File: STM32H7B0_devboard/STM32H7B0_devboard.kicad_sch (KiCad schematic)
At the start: 20 parts, among them SW1 SW_SPDT, U1 STM32H7B0VBT6, Y1 25MHz, Y2 32.768KHz

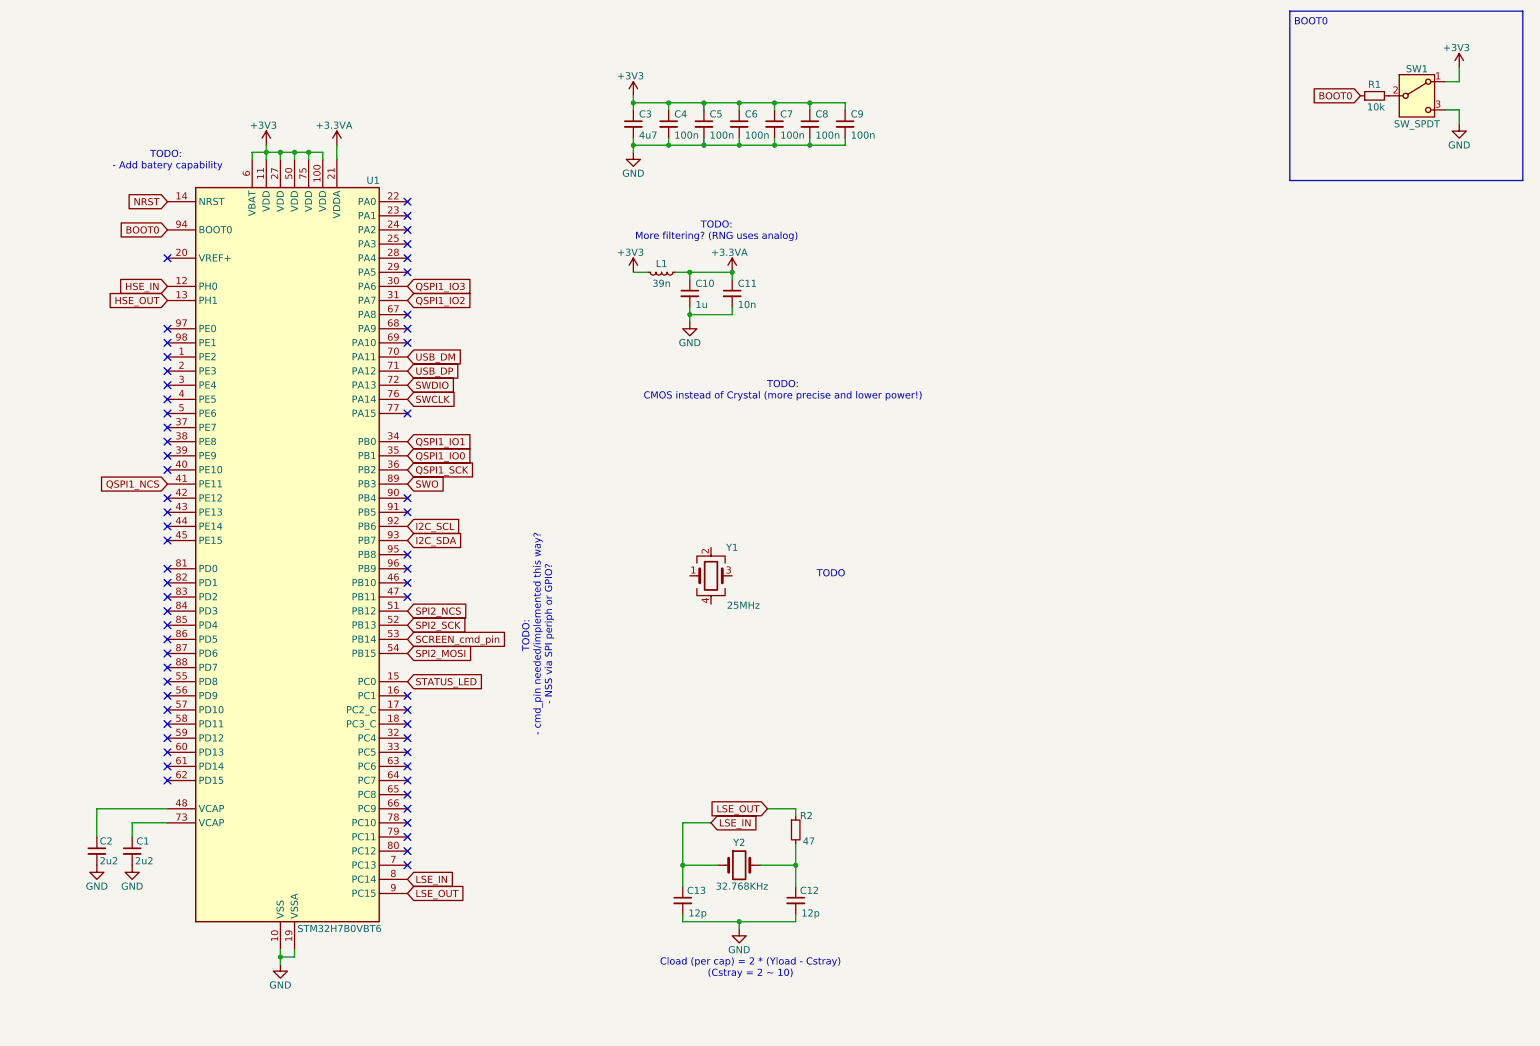
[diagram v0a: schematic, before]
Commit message: Schematic V0
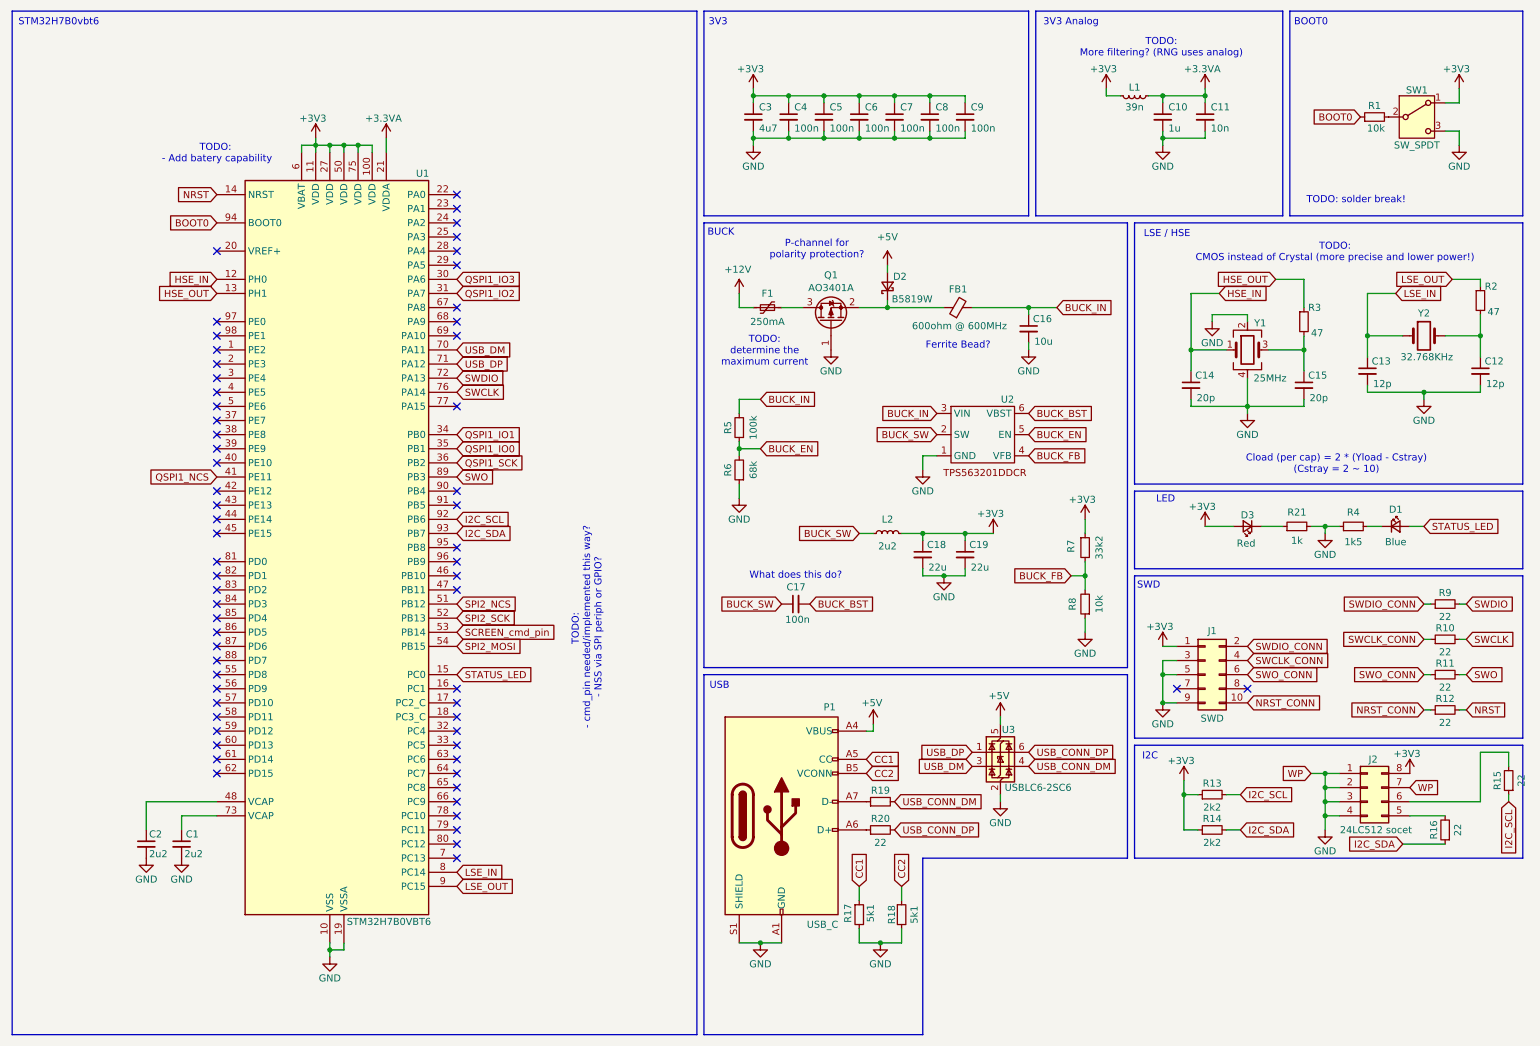
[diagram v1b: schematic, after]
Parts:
- added C14, C15: 20p, symbol Device:C_Small
- added C16: 10u, symbol Device:C_Small
- added C17: 100n, symbol Device:C_Small
- added C18, C19: 22u, symbol Device:C_Small
- added D1: Blue, symbol Device:LED_Small
- added D2: B5819W, symbol Device:D_Schottky_Small
- added D3: Red, symbol Device:LED_Small
- added F1: 250mA, symbol Device:Polyfuse_Small
- added FB1: 600ohm @ 600MHz, symbol Device:FerriteBead_Small
- added J1: SWD, symbol Connector_Generic:Conn_02x05_Odd_Even
- added J2: 24LC512 socet, symbol Connector_Generic:Conn_02x04_Counter_Clockwise
- added L2: 2u2, symbol Device:L_Small
- added P1: USB_C, symbol Connector:USB_C_Plug_USB2.0
- added Q1: AO3401A, Package_TO_SOT_SMD:SOT-23, symbol Transistor_FET:AO3401A
- added R10, R11, R12, R15, R16, R19, R20, R9: 22, symbol Device:R_Small
- added R13, R14: 2k2, symbol Device:R_Small
- added R17, R18: 5k1, symbol Device:R_Small
- added R21: 1k, symbol Device:R_Small
- added R3: 47, symbol Device:R_Small
- added R4: 1k5, symbol Device:R_Small
- added R5: 100k, symbol Device:R_Small
- added R6: 68k, symbol Device:R_Small
- added R7: 33k2, symbol Device:R_Small
- added R8: 10k, symbol Device:R_Small
- added U2: ~, symbol Marijn:TPS563201DDCR
- added U3: USBLC6-2SC6, Package_TO_SOT_SMD:SOT-23-6, symbol Power_Protection:USBLC6-2SC6
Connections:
- net +3V3: now also C18.1, C19.1, D3.2 (A), J1.1 (Pin_1), J2.8 (Pin_8), L2.2, R13.1, R14.1, R7.1
- net GND: now also Y1.2, Y1.4, C14.2, C15.2, C16.2, C18.2, C19.2, J1.3 (Pin_3), J1.5 (Pin_5), J1.9 (Pin_9), J2.1 (Pin_1), J2.2 (Pin_2), J2.3 (Pin_3), J2.4 (Pin_4), J2.7 (Pin_7), P1.A1 (GND), P1.A12 (GND), P1.B1 (GND), P1.B12 (GND), P1.S1 (SHIELD), Q1.1 (G), R17.2, R18.2, R21.2, R4.1, R6.1, R8.1, U2.1 (GND), U3.2 (GND)
- net HSE_IN: now also Y1.1, C14.1
- net HSE_OUT: now also R3.1
- net I2C_SCL: now also R13.2, R15.1
- net I2C_SDA: now also R14.2, R16.1
- net NRST: now also R12.2
- net STATUS_LED: now also D1.2 (A)
- net SWCLK: now also R10.2
- net SWDIO: now also R9.2
- net SWO: now also R11.2
- net USB_DM: now also U3.3 (I/O2)
- net USB_DP: now also U3.1 (I/O1)
- net at Y1.3: now also C15.1, R3.2
- new net: P1.A6 (D+), R20.1
- new net: P1.A7 (D-), R19.1
- new net: D2.1 (K), FB1.1, Q1.2 (S)
- new net: D3.1 (K), R21.1
- new net: F1.2, Q1.3 (D)
- new net: J2.5 (Pin_5), R16.2
- new net: J2.6 (Pin_6), R15.2
- new net: D1.1 (K), R4.2
- new net +12V: F1.1
- new net +5V: D2.2 (A), P1.A4 (VBUS), P1.A9 (VBUS), P1.B4 (VBUS), P1.B9 (VBUS), U3.5 (VBUS)
- new net BUCK_BST: C17.2, U2.6 (VBST)
- new net BUCK_EN: R5.1, R6.2, U2.5 (EN)
- new net BUCK_FB: R7.2, R8.2, U2.4 (VFB)
- new net BUCK_IN: C16.1, FB1.2, R5.2, U2.3 (VIN)
- new net BUCK_SW: C17.1, L2.1, U2.2 (SW)
- new net CC1: P1.A5 (CC), R17.1
- new net CC2: P1.B5 (VCONN), R18.1
- new net NRST_CONN: J1.10 (Pin_10), R12.1
- new net SWCLK_CONN: J1.4 (Pin_4), R10.1
- new net SWDIO_CONN: J1.2 (Pin_2), R9.1
- new net SWO_CONN: J1.6 (Pin_6), R11.1
- new net USB_CONN_DM: R19.2, U3.4 (I/O2)
- new net USB_CONN_DP: R20.2, U3.6 (I/O1)
- no-connect marks 61 -> 63
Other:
- note added: "3V3"
- note added: "3V3 Analog"
- note added: "BUCK"
- note added: "Ferrite Bead?"
- note added: "I2C"
- note added: "LED"
- note added: "LSE / HSE"
- note added: "P-channel for polarity protection?"
- note added: "STM32H7B0vbt6"
- note added: "SWD"
- note added: "TODO: determine the maximum current"
- note added: "TODO: solder break!"
- note added: "USB"
- note added: "What does this do?"
- note removed: "TODO"
- moved on the sheet: C1, C10, C11, C12, C13, C2, C3, C4, C5, C6, C7, C8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
